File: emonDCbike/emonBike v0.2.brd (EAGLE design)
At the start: 24.1 x 42.9 mm, 24 parts

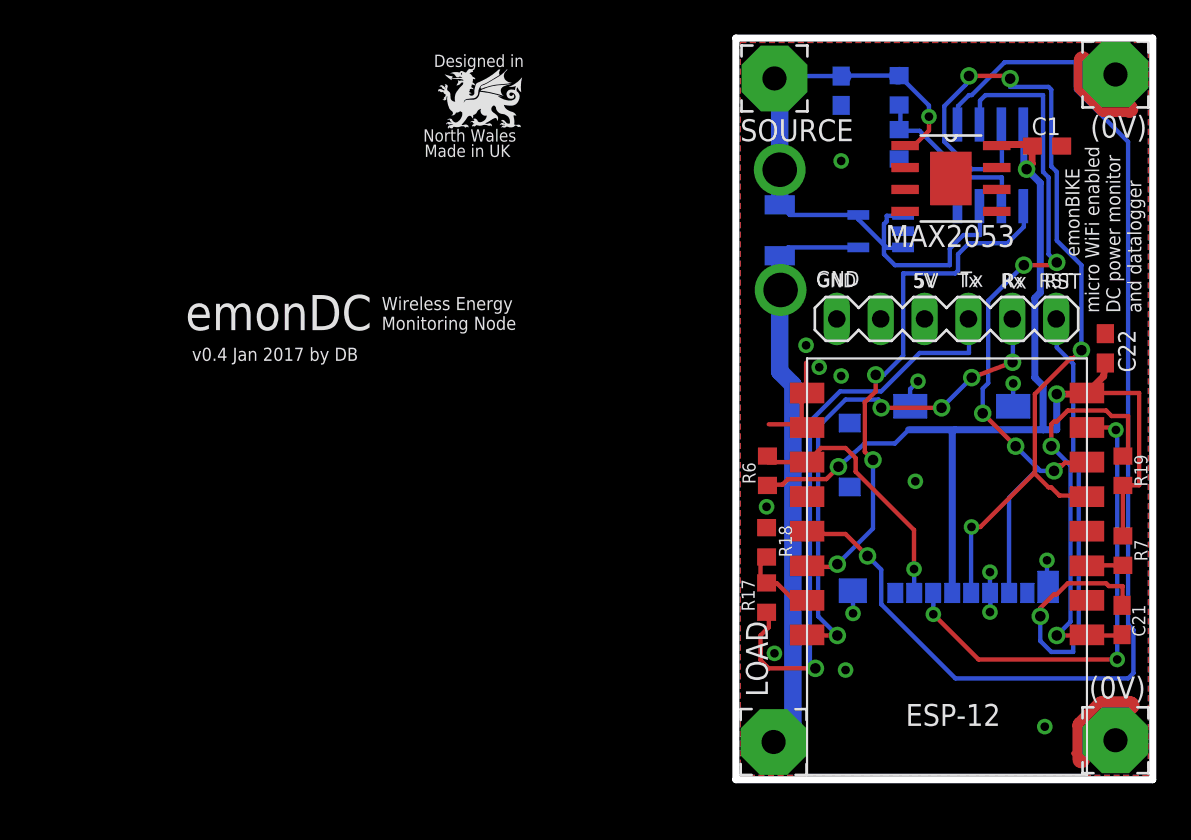
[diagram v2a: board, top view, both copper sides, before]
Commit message: tidy
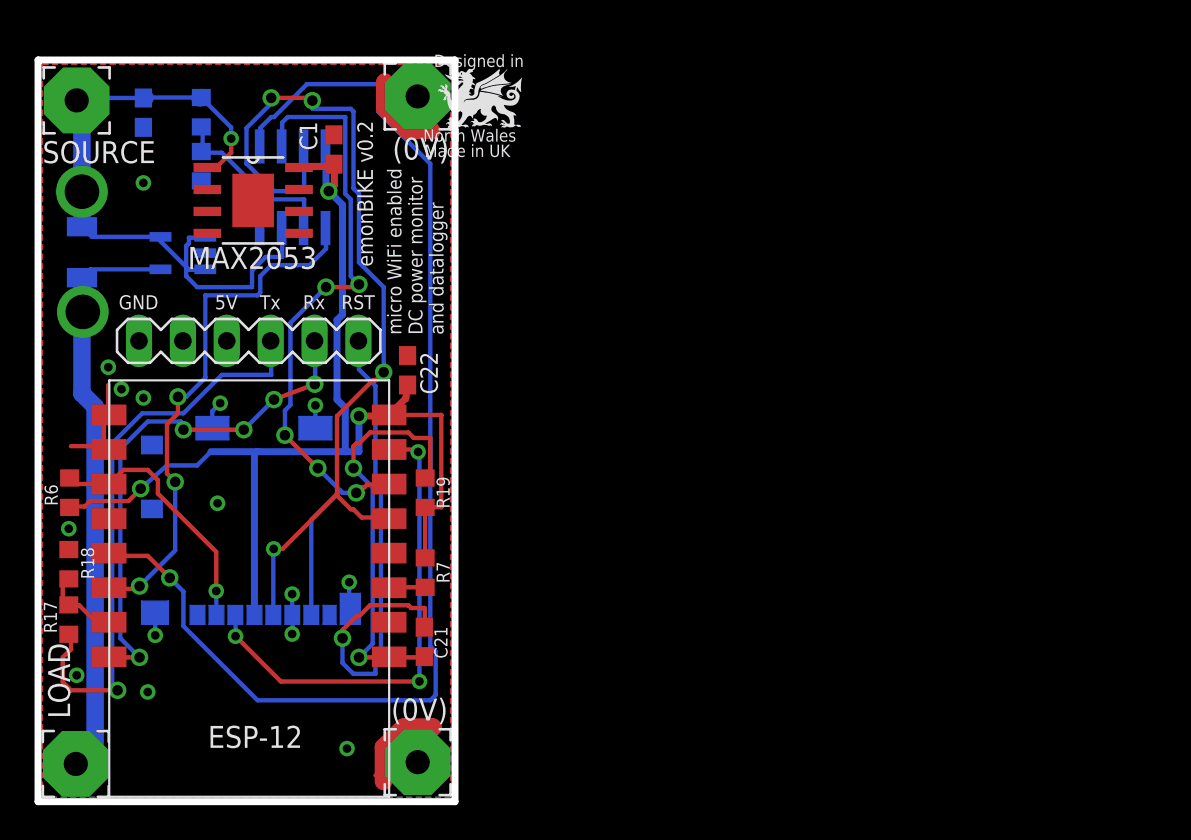
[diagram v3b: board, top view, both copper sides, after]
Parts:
- moved C1 41.3 mm to (18.6, 38.8), turned to 90 degrees
- moved C2 40.4 mm to (7.62, 40.9)
- moved LOGO1 40.4 mm to (15.0, 4.09)
- moved MAX2053 40.4 mm to (14.0, 35.8)
- moved MCP3002 40.4 mm to (16.3, 36.6)
- moved PAD1 40.4 mm to (3.71, 3.20)
- moved PAD2 40.4 mm to (3.76, 41.6)
- moved R17 40.4 mm to (3.30, 11.6)
- moved R18 40.4 mm to (3.30, 14.8)
- moved R2 40.4 mm to (11.0, 40.9)
- moved R3 40.4 mm to (11.0, 37.8)
- moved R_SENSE 40.4 mm to (4.06, 32.8)
- moved ZXCT1086 40.4 mm to (9.91, 32.8)
- moved C21 40.4 mm to (23.9, 10.3)
- moved C22 40.4 mm to (22.9, 26.0)
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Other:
- board text added: "emonBIKE v0.2"
- board text removed: "Wireless Energy Monitoring Node"
- board text removed: "emonBIKE"
- board text removed: "emonDC"
- board text removed: "v0.4 Jan 2017 by DB"
